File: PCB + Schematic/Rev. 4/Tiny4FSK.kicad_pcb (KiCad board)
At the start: 4 copper layers, 36.3 x 69.2 mm, 84 parts, among them J1 SWD, J2 GPIO, J3 USBC, J4 USB, J5 I2C, J6 Power Ext, J7 SPI, J8 USB Breakout, SW1 RST, SW2 Power Switch, U1 BME280, U2 ATGM336H, U3 SI4063, U4 ATSAMD21G18A-A, U5 1XZA032768AD19, U6 TPS61200DRC, U8 Linear Step-Down

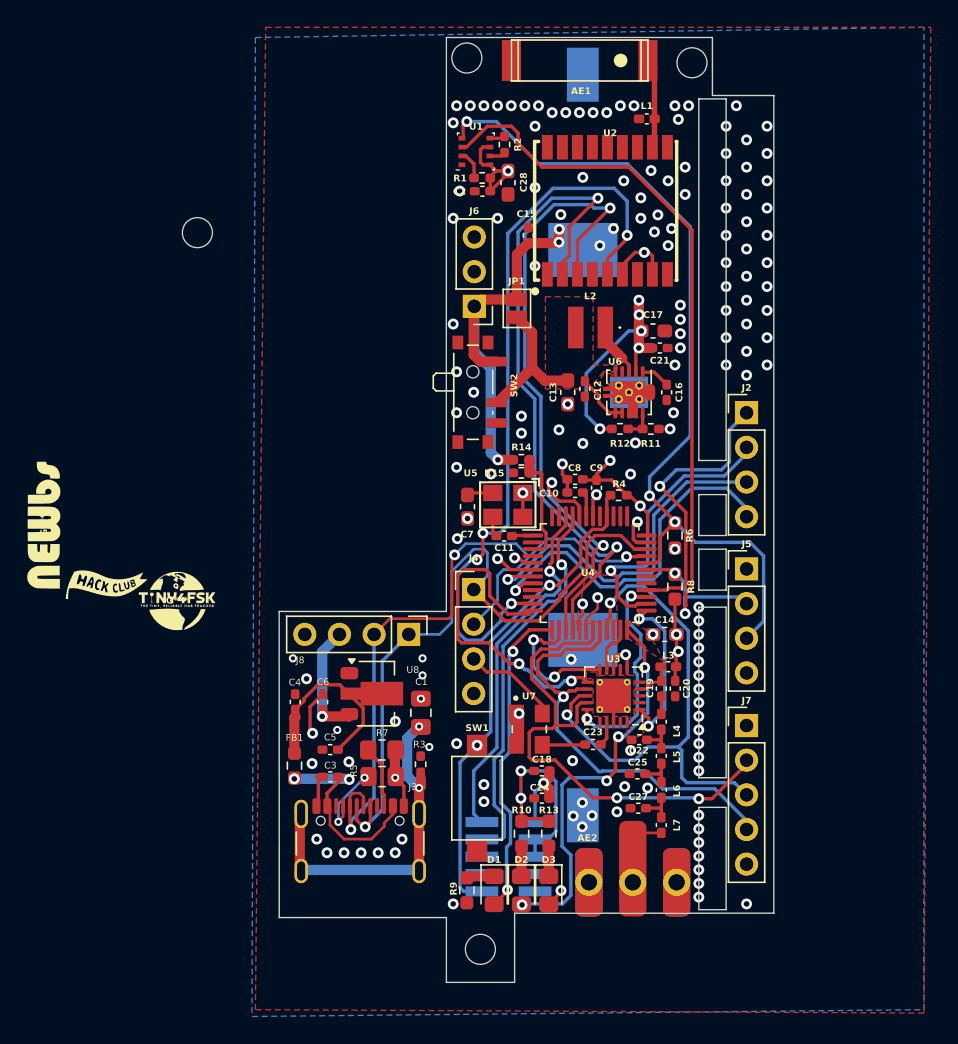
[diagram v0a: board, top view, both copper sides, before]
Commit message: JLCPCB optimization
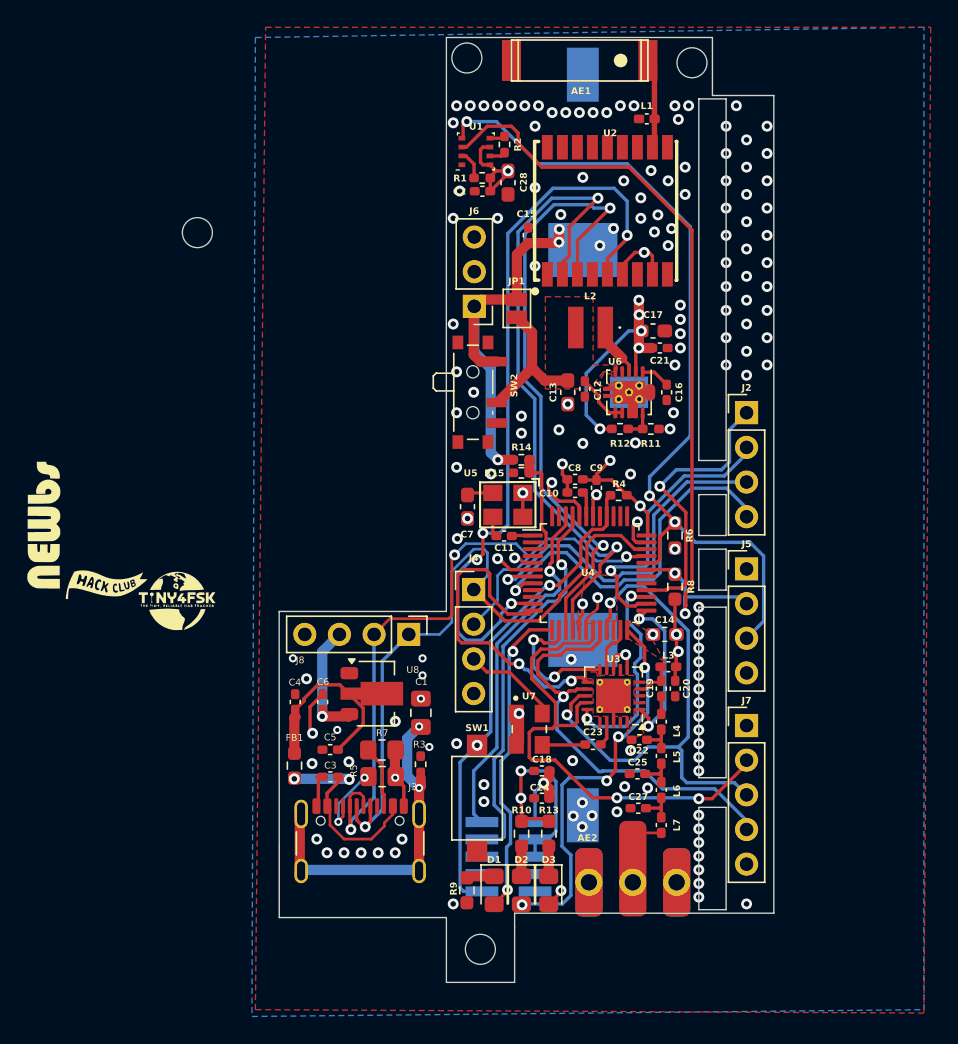
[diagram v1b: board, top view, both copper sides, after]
